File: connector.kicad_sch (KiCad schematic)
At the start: 1 part, among them J4 Conn_02x13_Row_Letter_Last

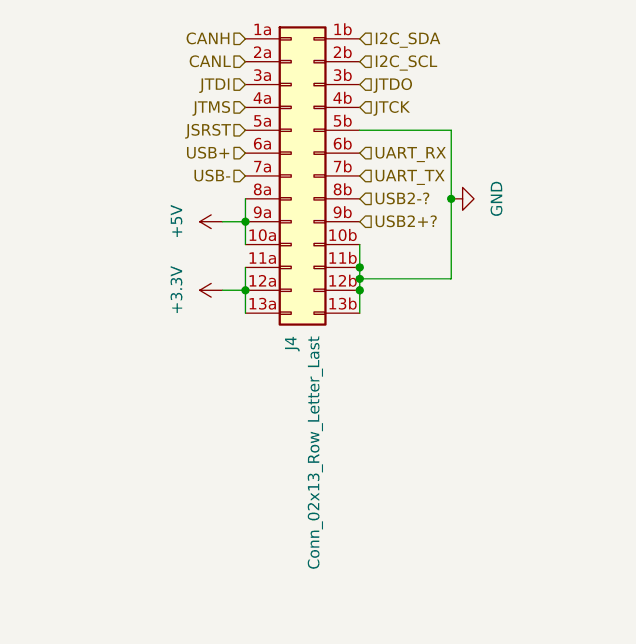
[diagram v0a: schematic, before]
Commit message: linked everything together. still need to add capacitors
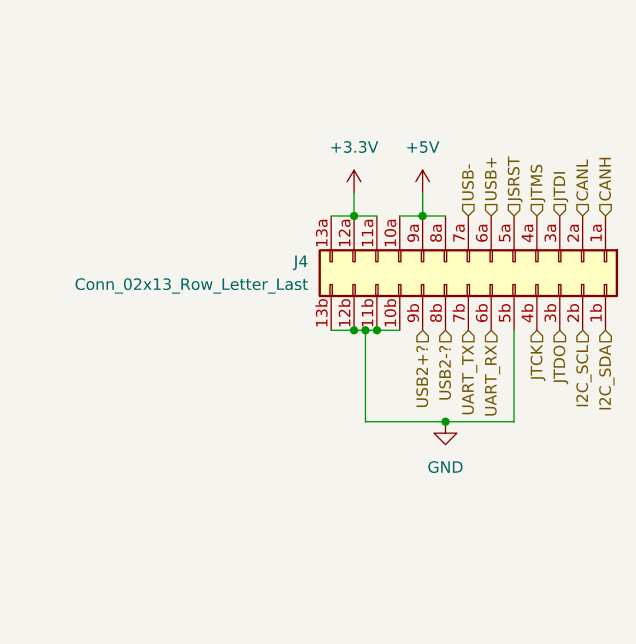
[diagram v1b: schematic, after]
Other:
- moved on the sheet: J4
